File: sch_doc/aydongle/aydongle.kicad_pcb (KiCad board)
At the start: 2 copper layers, 51 parts, among them J1 prog, J2 USB_A, J3 Display, J4 Audio-Jack-3, Q1 Q_Photo_NPN_EC, Q2 Q_Photo_NPN_CE, U1 AP1117-33, U2 STM32F103C8TxSmall, U3 YM2149F, U4 LM4811, Y1 12MHz

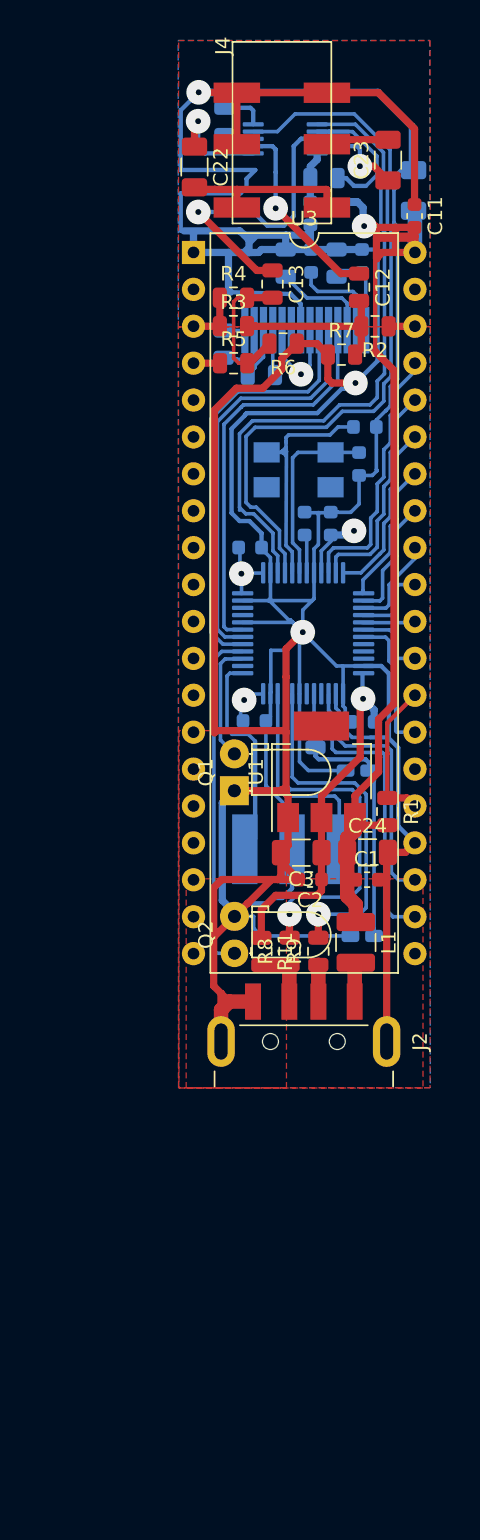
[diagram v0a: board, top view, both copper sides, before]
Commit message: ---
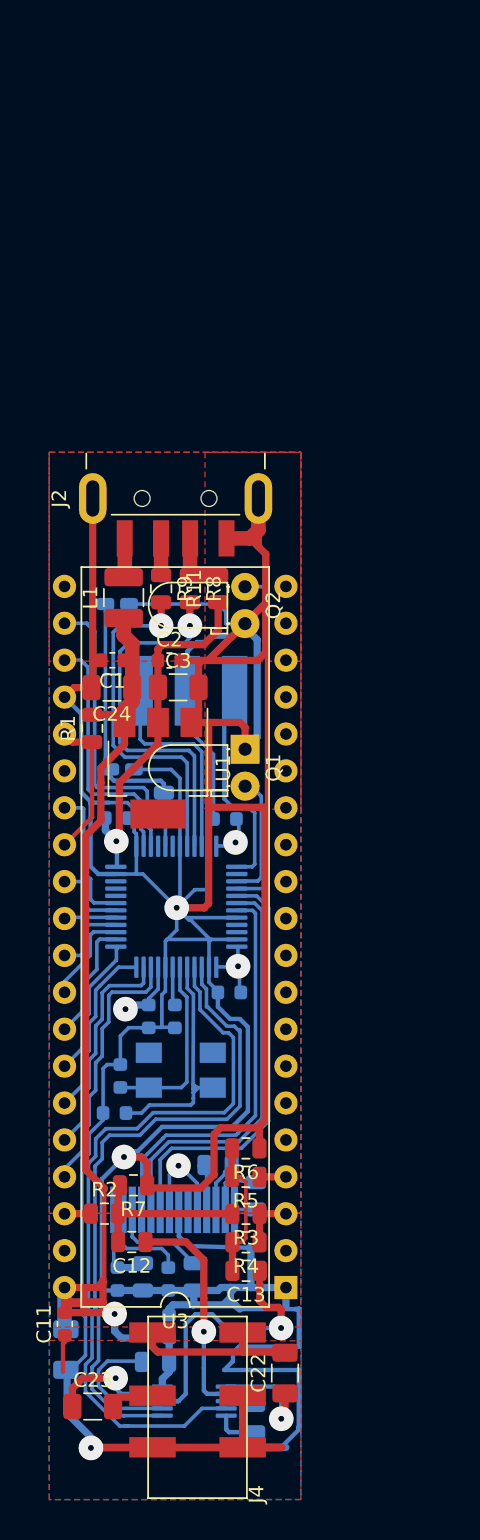
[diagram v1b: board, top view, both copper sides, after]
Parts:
- moved C21 89.3 mm to (100.1, 133.1), turned to 90 degrees
- moved C23 88.2 mm to (89.0, 132.2), turned to 0 degrees
- moved U4 87.1 mm to (96.0, 131.8), turned to 180 degrees
- moved J4 86.3 mm to (96.2, 131.5), turned to 270 degrees
- moved C14 83.3 mm to (87.1, 128.3), turned to 270 degrees
- moved C22 83.2 mm to (102.2, 129.9), turned to 90 degrees
- moved R12 82.3 mm to (93.3, 129.2), turned to 180 degrees
- moved C11 80.0 mm to (87.1, 126.5), turned to 90 degrees
- moved C20 77.2 mm to (94.2, 126.7), turned to 270 degrees
- moved C17 72.1 mm to (90.7, 123.4), turned to 90 degrees
- moved U3 71.5 mm to (102.3, 124.0), turned to 180 degrees
- moved C16 71.0 mm to (92.4, 123.3), turned to 90 degrees
- moved C15 70.8 mm to (94.2, 123.4), turned to 90 degrees
- moved R10 70.1 mm to (95.9, 123.3), turned to 270 degrees
- moved C13 67.9 mm to (99.5, 122.9), turned to 180 degrees
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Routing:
- net GND: track 395.3 -> 401.4 mm
- net Net-(C23-Pad1): track 6.56 -> 8.58 mm
- net Net-(C12-Pad1): track 13.3 -> 15.2 mm
- net Net-(C13-Pad1): track 21.0 -> 19.3 mm
- net Net-(C23-Pad2): track 4.33 -> 3.21 mm
- net /SWCLK: track 14.9 -> 15.7 mm
- net /A_CLK: track 49.8 -> 50.5 mm
- net +5V: track 83.0 -> 82.4 mm
- net /PHOT_R: track 9.27 -> 9.79 mm
